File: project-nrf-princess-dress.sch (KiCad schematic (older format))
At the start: 1 part

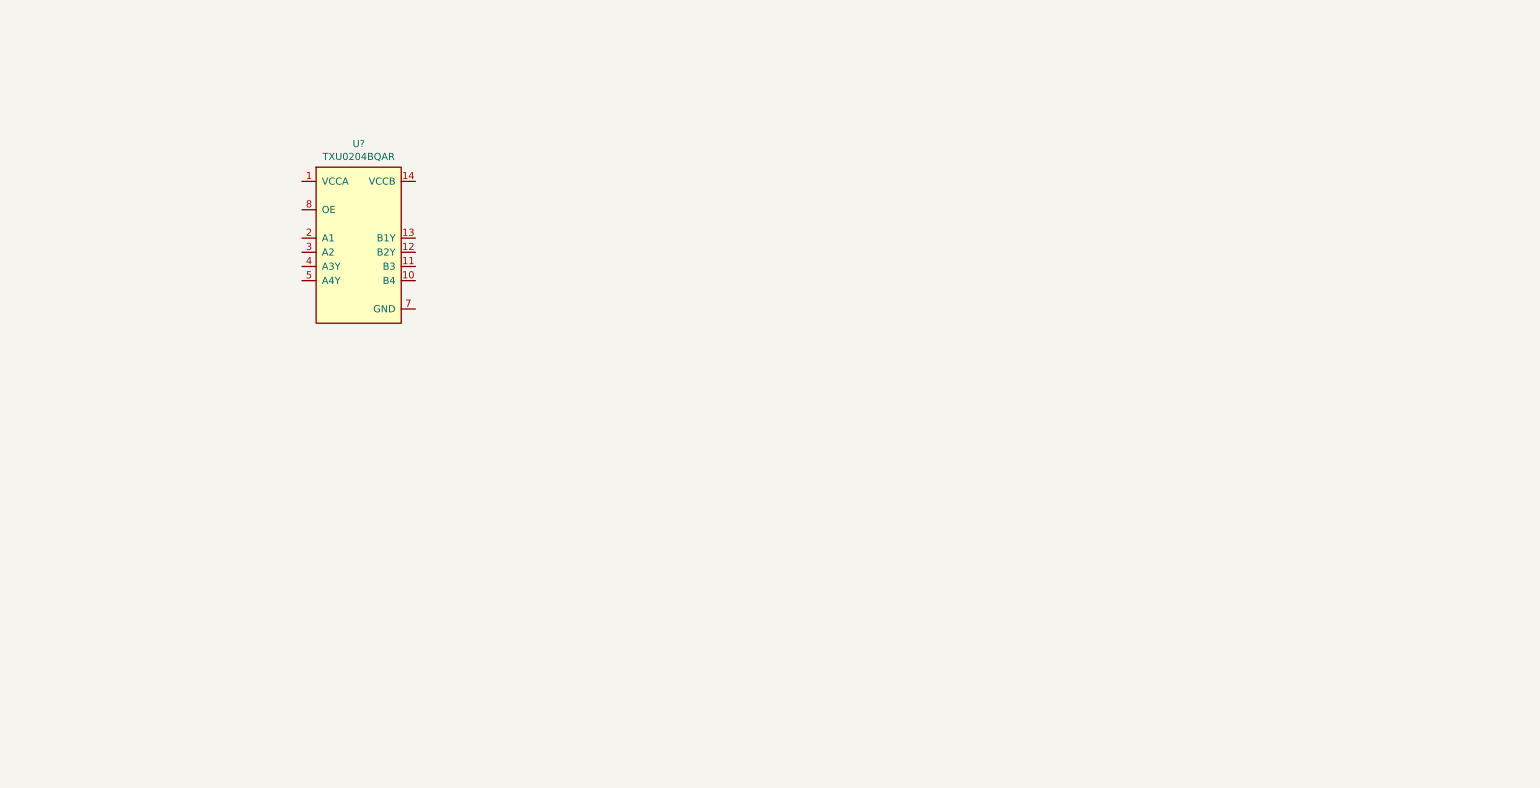
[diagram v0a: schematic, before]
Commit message: First schematic draft
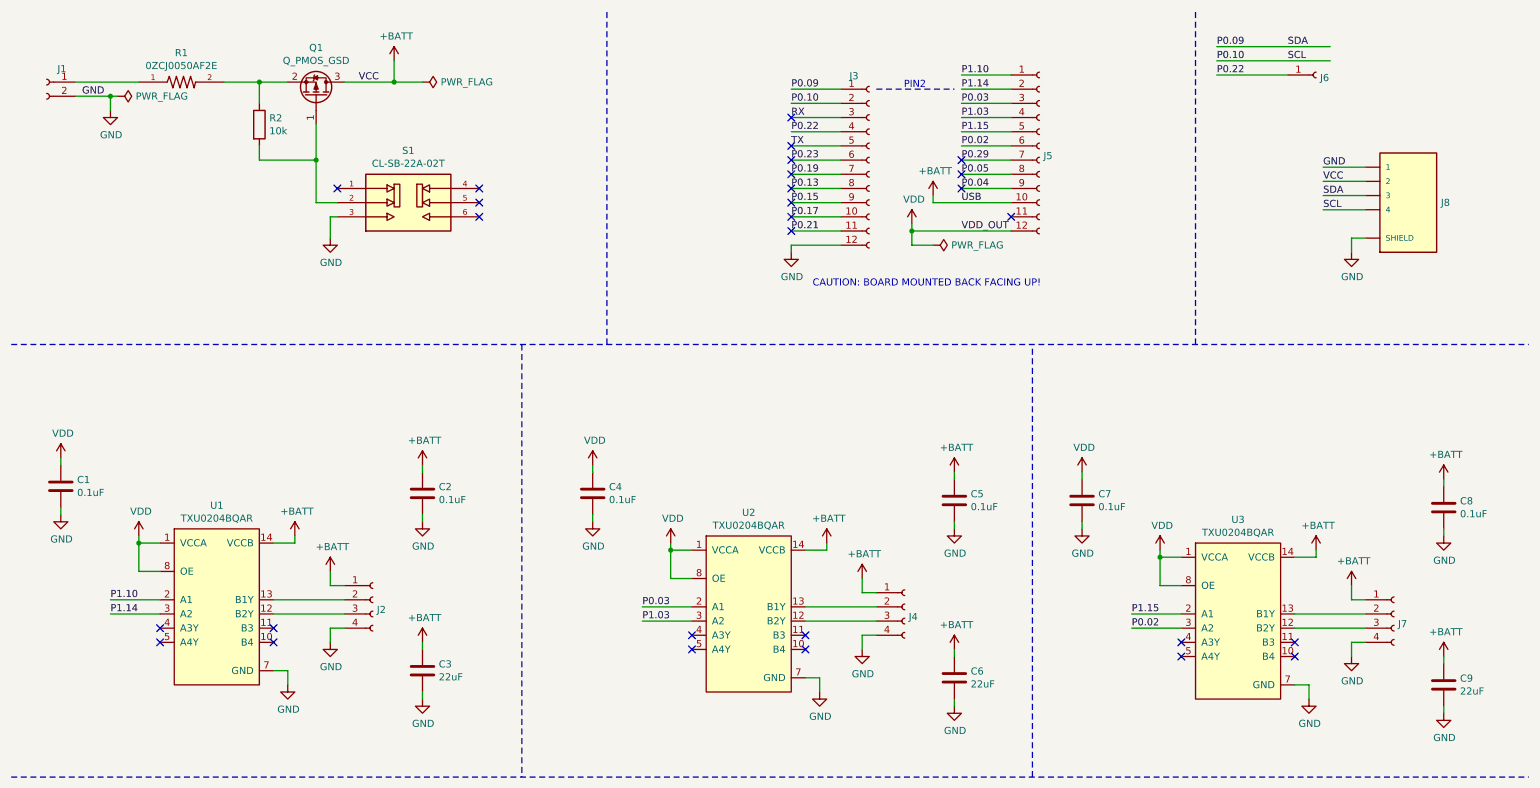
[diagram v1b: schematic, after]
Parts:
- added C1, C2, C4, C5, C7, C8: 0.1uF, Capacitor_SMD:C_0603_1608Metric, symbol Device:C
- added C3, C6, C9: 22uF, Capacitor_SMD:C_1210_3225Metric, symbol Device:C
- added J1: Conn_01x02_Female, TZ022101B000G:TZ022101B000G, symbol Connector:Conn_01x02_Female
- added J2, J4, J7: Conn_01x04_Female, TZ042101B000G:TZ042101B000G, symbol Connector:Conn_01x04_Female
- added J3, J5: Conn_01x12_Female, Connector_PinSocket_2.54mm:PinSocket_1x12_P2.54mm_Vertical_SMD_Pin1Right, symbol Connector:Conn_01x12_Female
- added J6: Conn_01x01_Female, Connector_Wire:SolderWirePad_1x01_SMD_5x10mm, symbol Connector:Conn_01x01_Female
- added J8: SM04B-SRSS-TB(LF)(SN), SM04B-SRSS-TB(LF)(SN):JST_SM04B-SRSS-TB(LF)(SN), symbol SM04B-SRSS-TB_LF__SN_:SM04B-SRSS-TB(LF)(SN)
- added Q1: Q_PMOS_GSD, Package_TO_SOT_SMD:SOT-23, symbol Device:Q_PMOS_GSD
- added R1: 0ZCJ0050AF2E, 0ZCJ0050AF2E:RESC3216X125N, symbol 0ZCJ0050AF2E:0ZCJ0050AF2E
- added R2: 10k, Resistor_SMD:R_0603_1608Metric, symbol Device:R
- added S1: CL-SB-22A-02T, CL-SB-22A-02T:SW_CL-SB-22A-02T, symbol CL-SB-22A-02T:CL-SB-22A-02T
- added U1, U2: TXU0204BQAR, TXU0204BQAR:TXU0204BQAR, symbol TXU0204BQAR:TXU0204BQAR
- gave numbers to parts that had none: 1
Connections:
- net VDD: now reaches U3.1 (VCCA)
- net VDD: now also U3.8 (OE), C1.1, C4.1, C7.1, J5.12 (Pin_12), U1.1 (VCCA), U1.8 (OE), U2.1 (VCCA), U2.8 (OE)
- net at U3.12 (B2Y): now also J7.3 (Pin_3)
- net at U3.13 (B1Y): now also J7.2 (Pin_2)
- net +BATT: now reaches U3.14 (VCCB)
- net +BATT: now also C2.1, C3.1, C5.1, C6.1, C8.1, C9.1, J2.1 (Pin_1), J4.1 (Pin_1), J5.10 (Pin_10), J7.1 (Pin_1), J8.2, Q1.3 (D), U1.14 (VCCB), U2.14 (VCCB)
- net P1.15: now reaches U3.2 (A1)
- net P1.15: now also J5.5 (Pin_5)
- net P0.02: now reaches U3.3 (A2)
- net P0.02: now also J5.6 (Pin_6)
- net GND: now reaches U3.7 (GND)
- net GND: now also C1.2, C2.2, C3.2, C4.2, C5.2, C6.2, C7.2, C8.2, C9.2, J1.2 (Pin_2), J2.4 (Pin_4), J3.12 (Pin_12), J4.4 (Pin_4), J7.4 (Pin_4), J8.1, J8.S1 (SHIELD), J8.S2 (SHIELD), S1.3, U1.7 (GND), U2.7 (GND)
- new net: J1.1 (Pin_1), R1.1
- new net: Q1.2 (S), R1.2, R2.1
- new net: Q1.1 (G), R2.2, S1.2
- new net: J4.3 (Pin_3), U2.12 (B2Y)
- new net: J4.2 (Pin_2), U2.13 (B1Y)
- new net: J2.3 (Pin_3), U1.12 (B2Y)
- new net: J2.2 (Pin_2), U1.13 (B1Y)
- new net P0.03: J5.3 (Pin_3), U2.2 (A1)
- new net P0.04: J5.9 (Pin_9)
- new net P0.05: J5.8 (Pin_8)
- new net P0.09: J3.1 (Pin_1), J8.3
- new net P0.10: J3.2 (Pin_2), J8.4
- new net P0.13: J3.8 (Pin_8)
- new net P0.15: J3.9 (Pin_9)
- new net P0.17: J3.10 (Pin_10)
- new net P0.19: J3.7 (Pin_7)
- new net P0.21: J3.11 (Pin_11)
- new net P0.22: J3.4 (Pin_4), J6.1 (Pin_1)
- new net P0.23: J3.6 (Pin_6)
- new net P0.29: J5.7 (Pin_7)
- new net P1.03: J5.4 (Pin_4), U2.3 (A2)
- new net P1.10: J5.1 (Pin_1), U1.2 (A1)
- new net P1.14: J5.2 (Pin_2), U1.3 (A2)
- new net RX: J3.3 (Pin_3)
- new net TX: J3.5 (Pin_5)
- no-connect marks 0 -> 28
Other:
- note added: "CAUTION: BOARD MOUNTED BACK FACING UP!"
- note added: "PIN2"
- moved on the sheet: U3
